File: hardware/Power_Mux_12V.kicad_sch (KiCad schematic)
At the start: 1 part

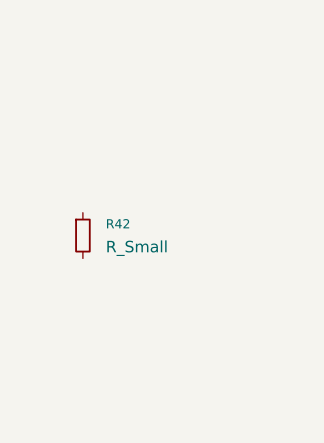
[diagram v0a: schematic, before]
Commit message: new contactor design block, started power mux
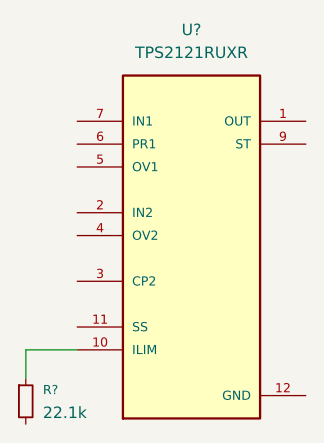
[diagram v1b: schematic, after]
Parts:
- removed R42: R_Small, symbol Device:R_Small
- added R?: 22.1k, symbol Device:R_Small
- added U?: TPS2121RUXR, LHRS_Power:IC_TPS2121RUXR, symbol lhrs_power:TPS2121RUXR
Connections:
- new net: R?.1, U?.10 (ILIM)
- new net: U?.1 (OUT), U?.1_1 (OUT), U?.8 (OUT), U?.8_1 (OUT)
- new net: U?.2 (IN2), U?.2_1 (IN2)
- new net: U?.7 (IN1), U?.7_1 (IN1)
